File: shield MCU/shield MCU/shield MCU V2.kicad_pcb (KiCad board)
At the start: 2 copper layers, 73.3 x 139.7 mm, 16 parts, among them J1 IR_sensor, J2 IR_sensor, J3 IR_sensor, J4 IR_sensor, J5 IR_sensor, J6 BATT, SW1 Pwr_Sw, U1 pwr_mgr_1, U3 gy50, U4 NUCLEO144-F429ZI

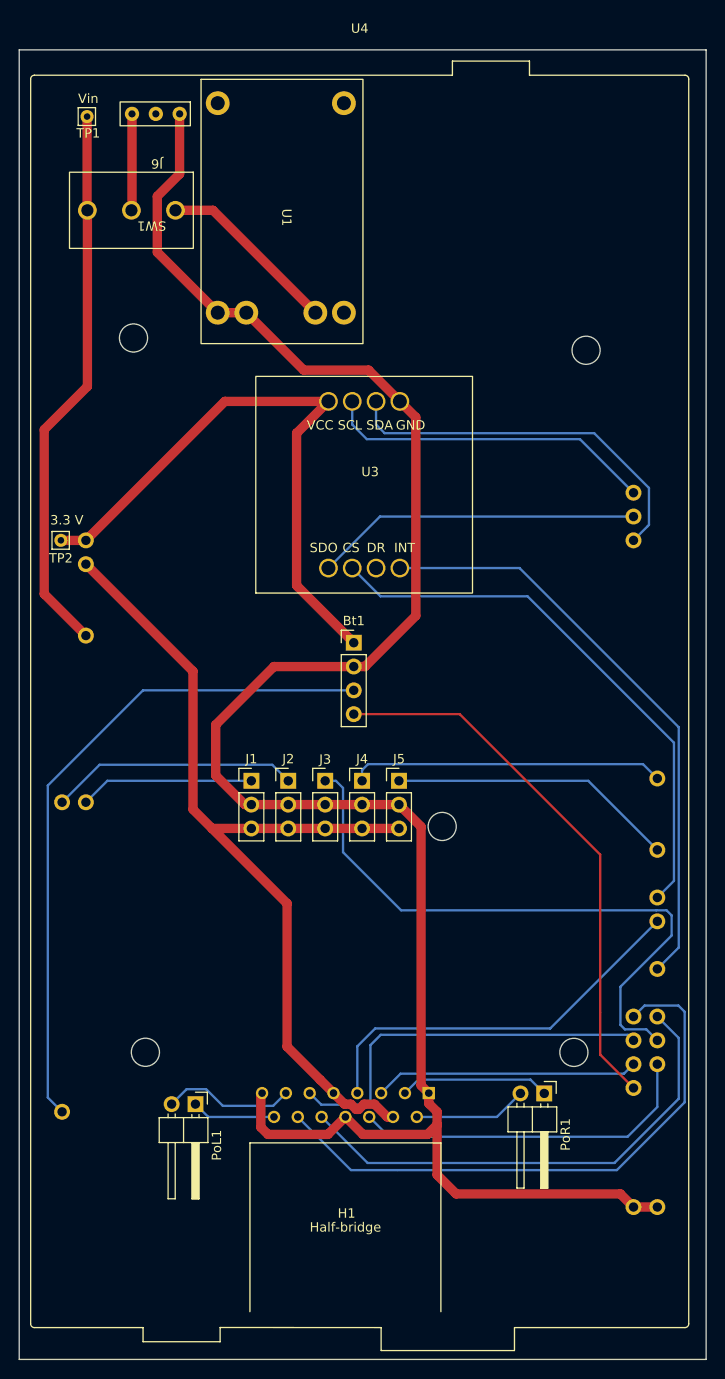
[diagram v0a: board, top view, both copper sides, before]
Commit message: uusi pcb
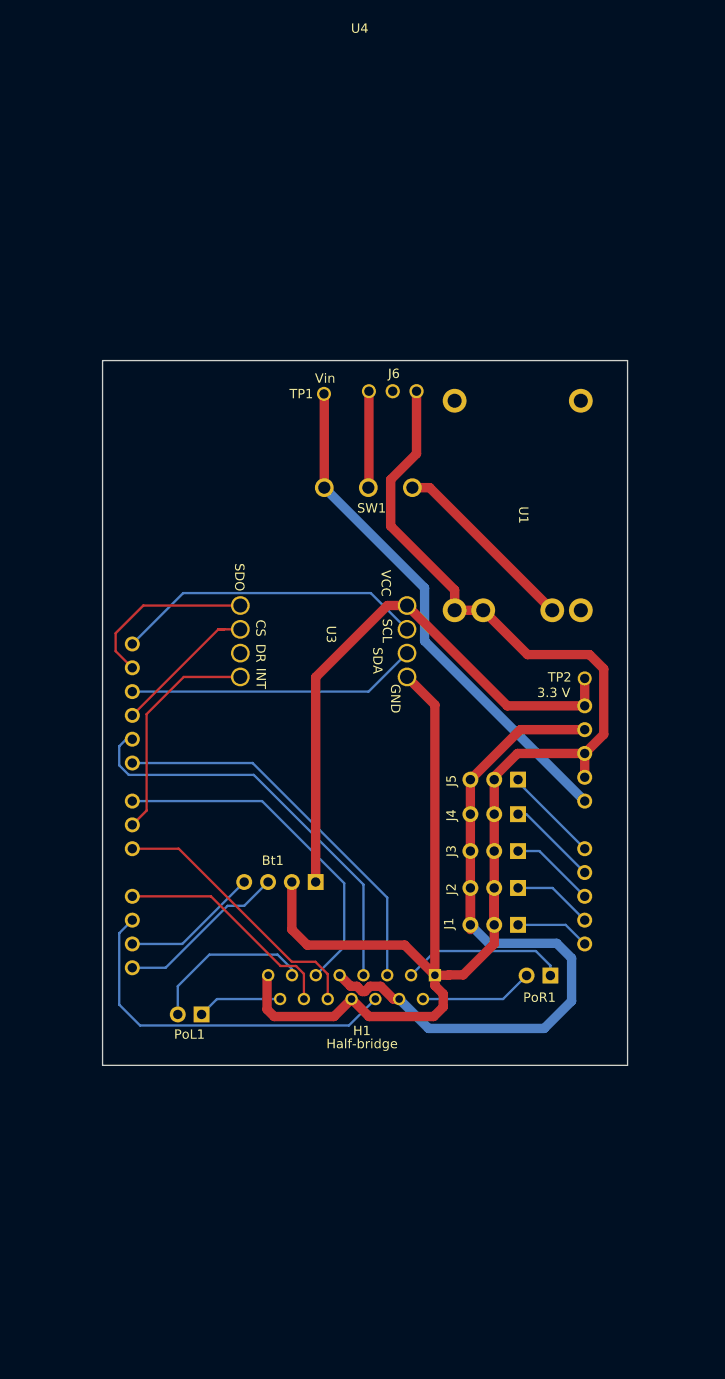
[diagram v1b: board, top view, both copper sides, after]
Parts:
- moved TP2 57.8 mm to (154.4, 99.8)
- moved U1 40.6 mm to (138.8, 67.7)
- moved SW1 38.9 mm to (138.0, 75.4)
- moved J6 38.9 mm to (137.6, 67.9)
- moved TP1 38.9 mm to (126.6, 69.5)
- moved J4 28.7 mm to (147.3, 114.3), turned to -90 degrees
- moved Bt1 25.8 mm to (125.7, 121.5), turned to -90 degrees
- moved J3 25.6 mm to (147.3, 118.2), turned to -90 degrees
- moved J2 23.5 mm to (147.3, 122.2), turned to -90 degrees
- moved J1 22.6 mm to (147.3, 126.1), turned to -90 degrees
- moved J5 12.7 mm to (147.3, 110.6), turned to -90 degrees
- moved PoR1 12.6 mm to (150.8, 131.5)
- moved H1 12.6 mm to (138.4, 131.5)
- moved PoL1 9.59 mm to (113.6, 135.7)
- moved U3 7.73 mm to (115.0, 84.3), turned to -90 degrees
- renumbered J4 to J1, J3 to J2, J2 to J3, J1 to J4
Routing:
- net Net-(J3-Pad1): track 65.5 -> 8.53 mm
- net Net-(Bt1-Pad3): track 72.3 -> 18.3 mm
- net Net-(Bt1-Pad4): track 58.9 -> 14.7 mm
- net Net-(U3-Pad2): track 59.3 -> 16.0 mm
- net Net-(U3-Pad4): track 63.5 -> 24.1 mm
- net Net-(H1-Pad12): track 62.5 -> 24.4 mm
- net GND: track 215.1 -> 182.3 mm
- net Net-(J4-Pad1): track 33.5 -> 7.95 mm
- net Net-(H1-Pad10): track 52.7 -> 29.0 mm
- net Net-(U4-Pad114): track 30.6 -> 10.3 mm
- net Net-(J2-Pad1): track 26.5 -> 9.11 mm
- net Net-(U3-Pad1): track 34.8 -> 19.0 mm
- net /5V: track 95.2 -> 79.4 mm
- net Net-(H1-Pad5): track 28.2 -> 41.4 mm
- net Net-(U3-Pad7): track 40.7 -> 31.0 mm
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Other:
- board size 73.3 x 139.7 mm -> 56 x 75.2 mm
